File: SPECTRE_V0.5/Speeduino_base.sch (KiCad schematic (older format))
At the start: 191 parts, among them J1 Conn_01x04_Male, J2 Conn_02x04_Odd_Even, J3 Conn_01x06_Male, Q1 2N7002, Q10 BSP78, Q11 BSP78, Q12 BSP78, Q13 BSP78, Q14 BSP78, Q15 BSP78, Q16 BSP78, Q17 BSP78, Q18 BSP78, Q19 SMD-MOSFET-N-CH-30V-5.8A-AO34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, Q2 CJ2302, Q20 AO3401A, Q3 CJ2302, Q4 CJ2302, Q5 BSP78, Q6 BSP78, Q7 CJ2302, Q8 CJ2302, Q9 CJ2302, U1 MAX9926UAEE+, U2 molex_48pin, U3 LM78M05_TO220, U4 MAX3232

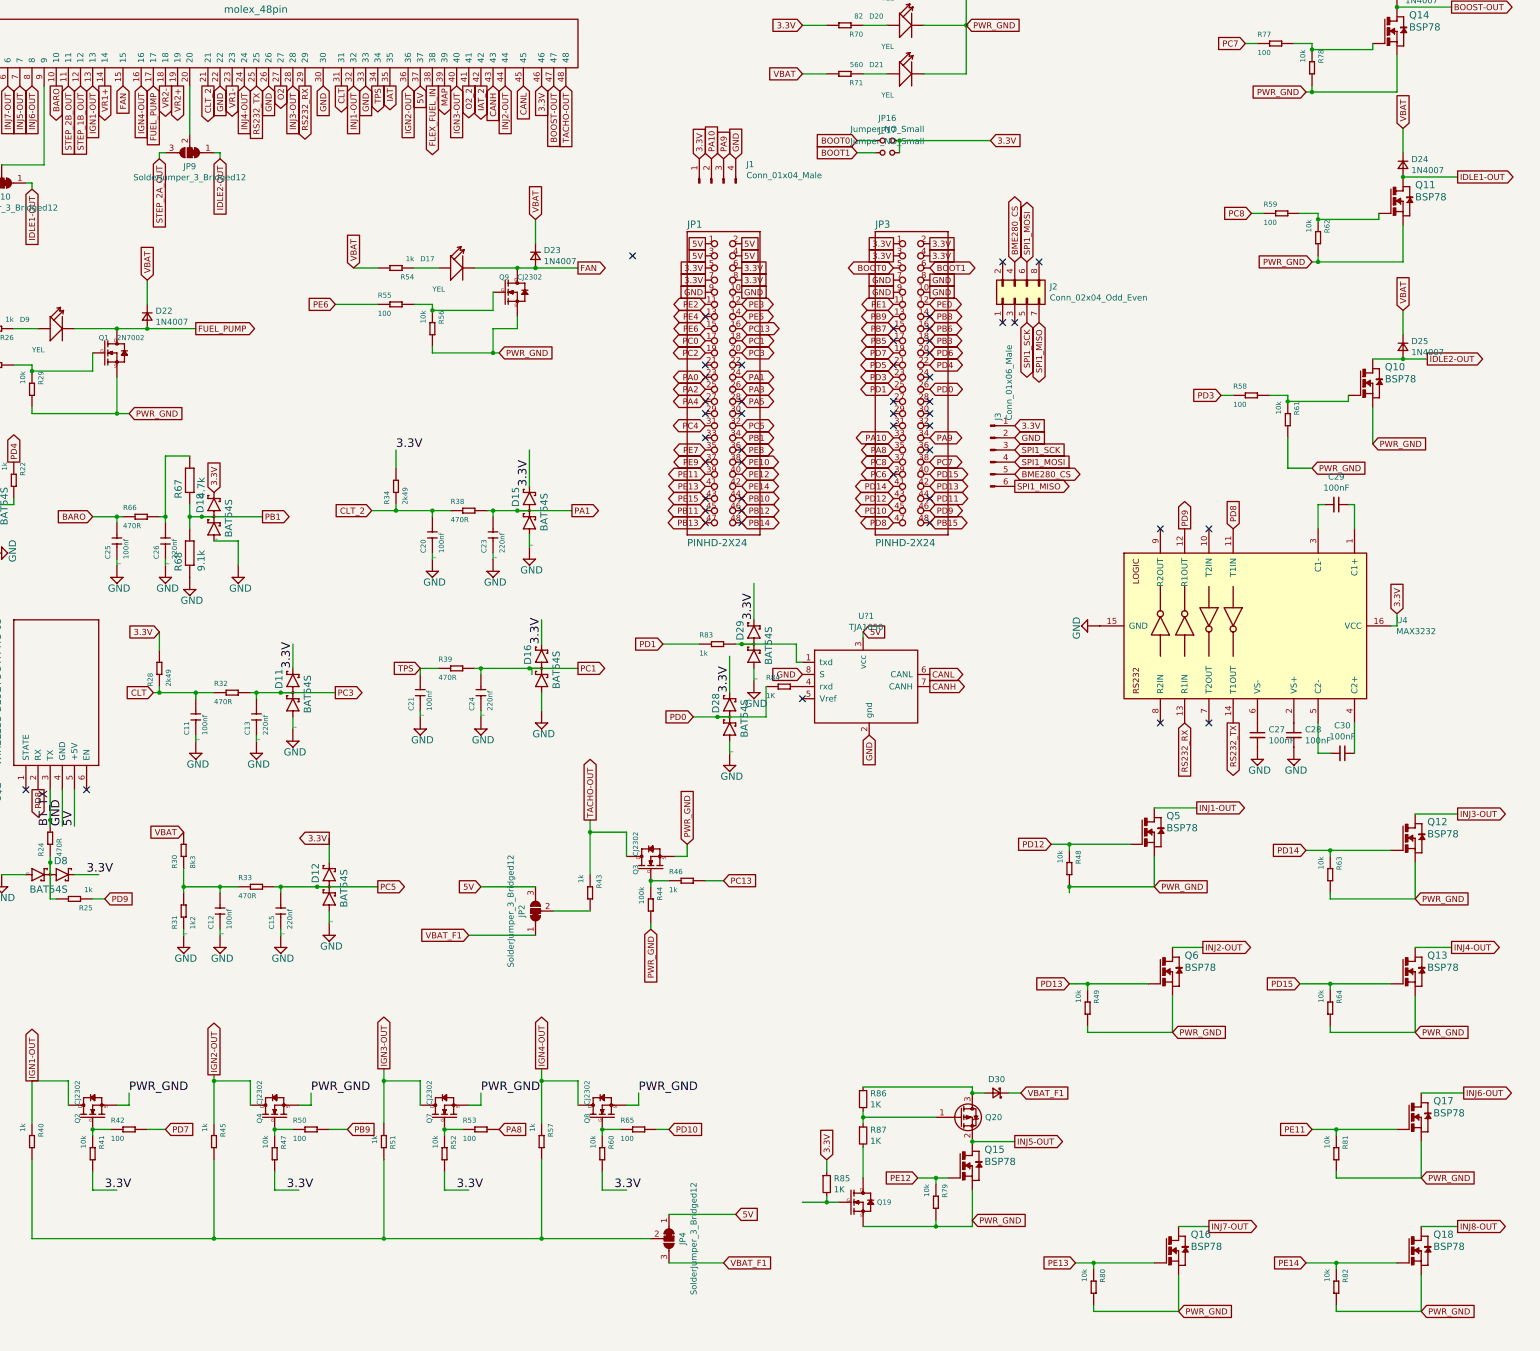
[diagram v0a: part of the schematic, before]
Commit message: Routing V0.5
Started routing board V0.5
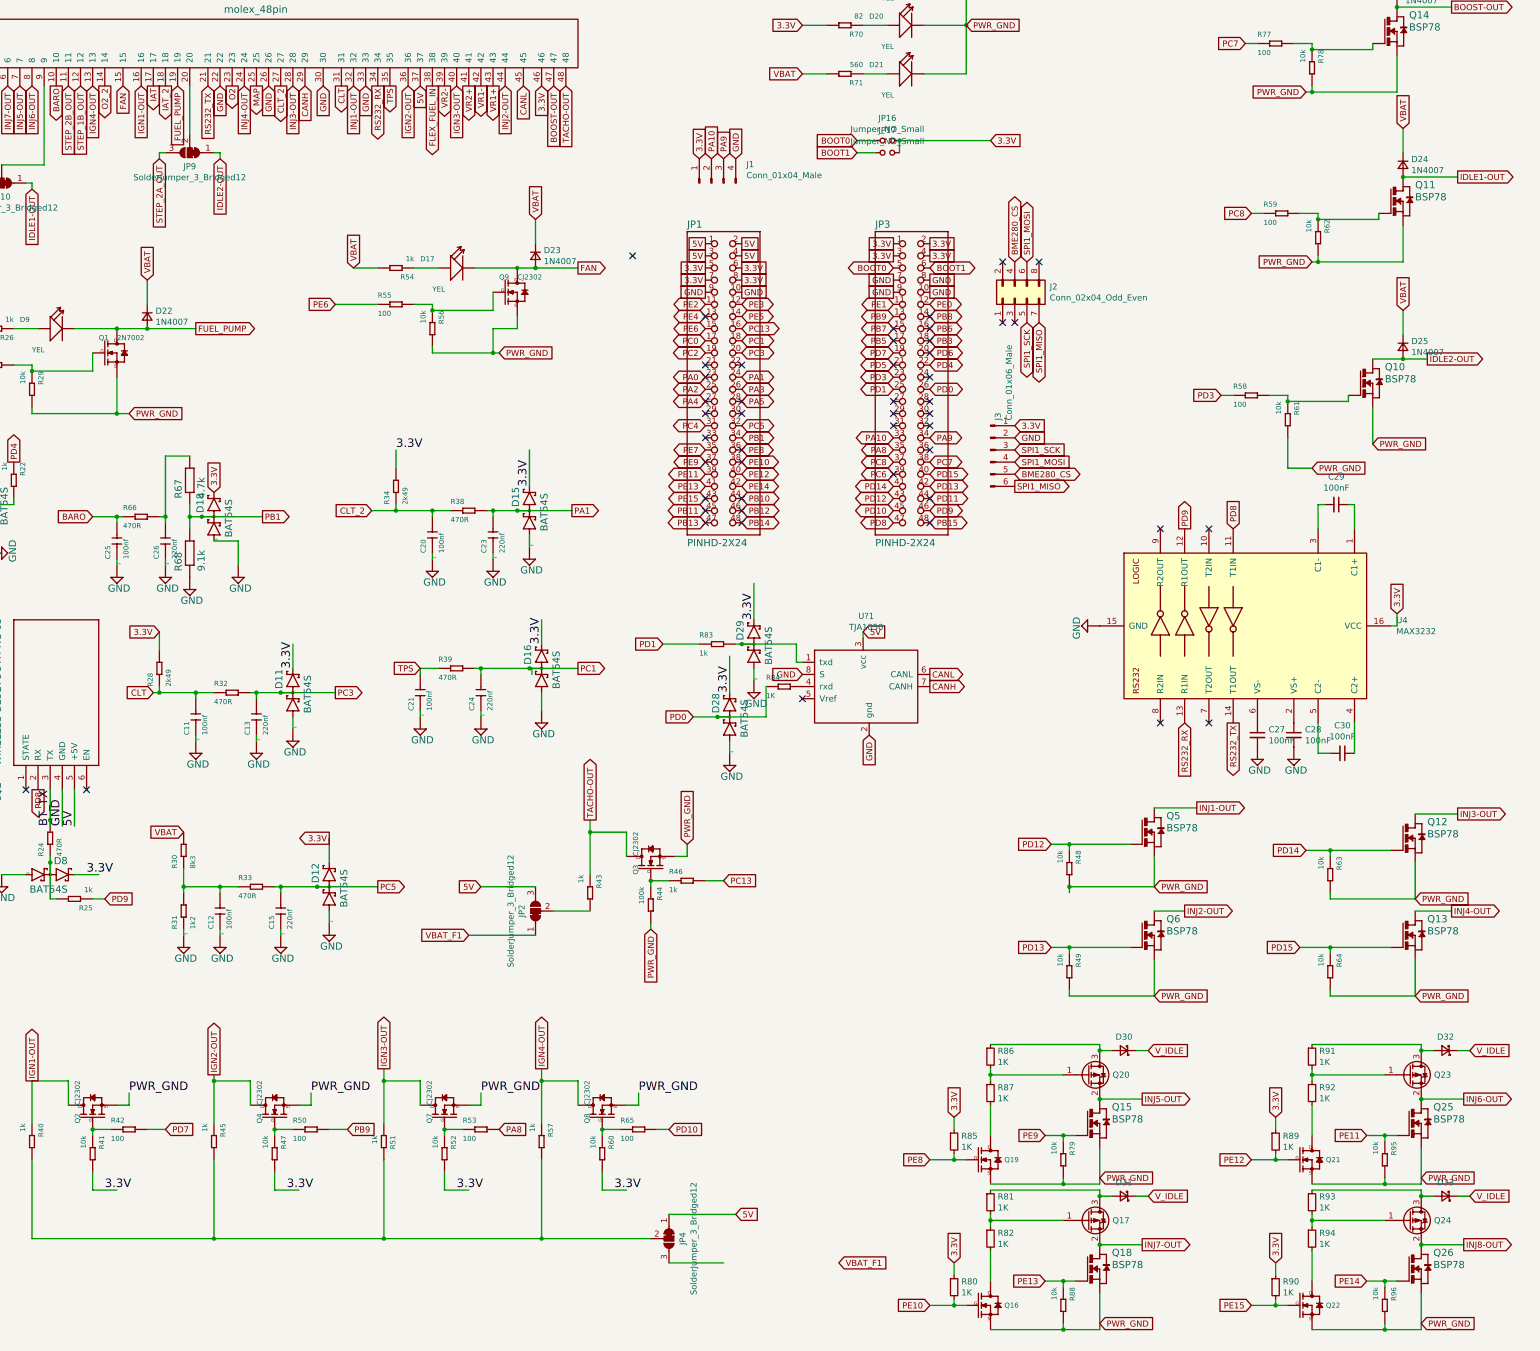
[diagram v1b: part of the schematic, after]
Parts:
- removed Q16, Q17: BSP78, Speeduino_base:SOT223, symbol Speeduino_base-eagle-import:NMOSSOT223
- removed R80, R81, R82: 10k, Speeduino_base:R0603, symbol Speeduino_base-eagle-import:SMD-RES-470R-5%-1_10W(0603)
- added D31, D32, D33: SS310, Diode_SMD:D_SMA, symbol Device:D_Schottky_Small
- added Q16, Q21, Q22: SMD-MOSFET-N-CH-30V-5.8A-AO3400(SOT-23), Package_TO_SOT_SMD:SOT-23_Handsoldering, symbol speeduino_lib:SMD-MOSFET-N-CH-30V-5.8A-AO3400(SOT-23)
- added Q17, Q23, Q24: AO3401A, Package_TO_SOT_SMD:SOT-23_Handsoldering, symbol Transistor_FET:AO3401A
- added Q25, Q26: BSP78, Speeduino_base:SOT223, symbol Speeduino_base-eagle-import:NMOSSOT223
- added R80, R81, R82, R89, R90, R91, R92, R93, R94: 1K, Speeduino_base:R_0603_1608Metric_Pad1.05x0.95mm_HandSolder, symbol Device:R_Small
- added R88, R95, R96: 10k, Speeduino_base:R_0603_1608Metric_Pad1.05x0.95mm_HandSolder, symbol Speeduino_base-eagle-import:SMD-RES-470R-5%-1_10W(0603)
- Q20: footprint Package_TO_SOT_SMD:SOT-23 -> Package_TO_SOT_SMD:SOT-23_Handsoldering
- R79: footprint Speeduino_base:R0603 -> Speeduino_base:R_0603_1608Metric_Pad1.05x0.95mm_HandSolder
- R85, R86, R87: footprint Resistor_SMD:R_0603_1608Metric_Pad1.05x0.95mm_HandSolder -> Speeduino_base:R_0603_1608Metric_Pad1.05x0.95mm_HandSolder
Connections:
- wire segments 515 -> 554
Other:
- moved on the sheet: D30, Q13, Q15, Q19, Q20, Q6, R49, R64, R79, R85, R86, R87
